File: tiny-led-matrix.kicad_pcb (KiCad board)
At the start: 4 copper layers, 37.5 x 21.2 mm, 166 parts, among them J1 TagConnect_TC2030_SWD, U1 STM32F030F4Px

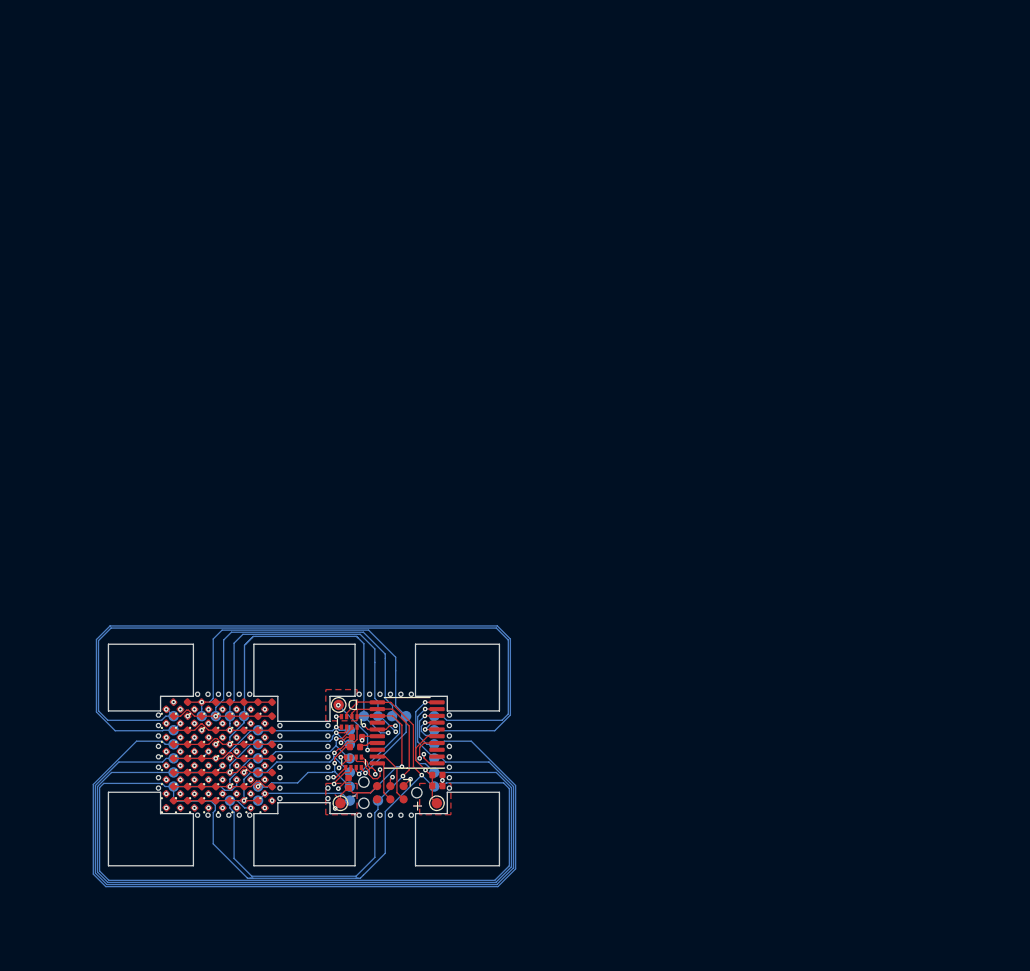
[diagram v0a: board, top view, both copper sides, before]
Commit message: Full panel
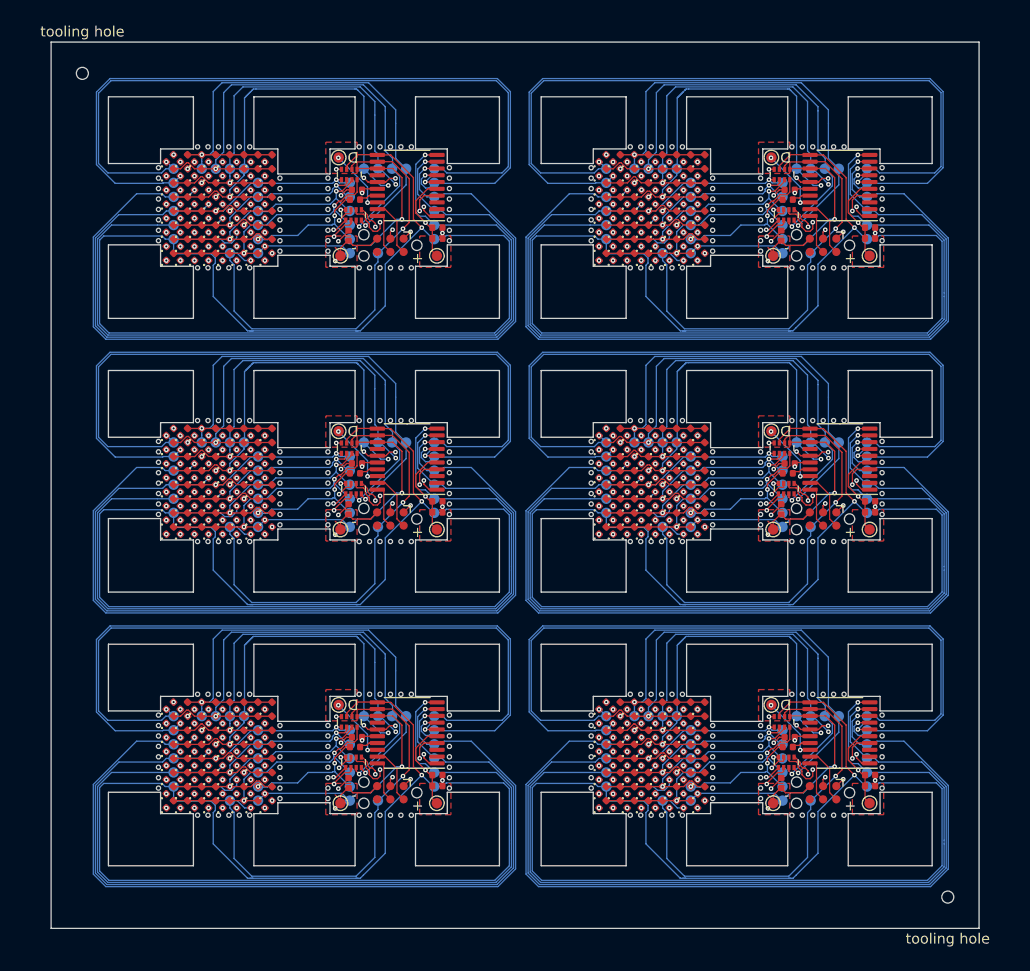
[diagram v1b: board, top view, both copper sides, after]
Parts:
- added C1: 10uF, Capacitor_SMD:C_0402_1005Metric, F.Cu at (167.2, 81.5)
- added C1: 10uF, Capacitor_SMD:C_0402_1005Metric, F.Cu at (167.2, 55.2)
- added C1: 10uF, Capacitor_SMD:C_0402_1005Metric, F.Cu at (167.2, 107.7)
- added C1: 10uF, Capacitor_SMD:C_0402_1005Metric, F.Cu at (125.7, 55.2)
- added C1: 10uF, Capacitor_SMD:C_0402_1005Metric, F.Cu at (125.7, 81.5)
- added C2: 100nF, Capacitor_SMD:C_0402_1005Metric, F.Cu at (159.4, 76.8)
- added C2: 100nF, Capacitor_SMD:C_0402_1005Metric, F.Cu at (159.4, 50.5)
- added C2: 100nF, Capacitor_SMD:C_0402_1005Metric, F.Cu at (159.4, 103.0)
- added C2: 100nF, Capacitor_SMD:C_0402_1005Metric, F.Cu at (117.9, 50.5)
- added C2: 100nF, Capacitor_SMD:C_0402_1005Metric, F.Cu at (117.9, 76.8)
- added C3: 100nF, Capacitor_SMD:C_0402_1005Metric, F.Cu at (167.2, 54.1)
- added C3: 100nF, Capacitor_SMD:C_0402_1005Metric, F.Cu at (167.2, 80.4)
- added C3: 100nF, Capacitor_SMD:C_0402_1005Metric, F.Cu at (167.2, 106.7)
- added C3: 100nF, Capacitor_SMD:C_0402_1005Metric, F.Cu at (125.7, 54.1)
- added C3: 100nF, Capacitor_SMD:C_0402_1005Metric, F.Cu at (125.7, 80.4)
- added C4: 100nF, Capacitor_SMD:C_0402_1005Metric, F.Cu at (158.6, 81.2)
- added C4: 100nF, Capacitor_SMD:C_0402_1005Metric, F.Cu at (158.6, 54.9)
- added C4: 100nF, Capacitor_SMD:C_0402_1005Metric, F.Cu at (158.6, 107.4)
- added C4: 100nF, Capacitor_SMD:C_0402_1005Metric, F.Cu at (117.1, 54.9)
- added C4: 100nF, Capacitor_SMD:C_0402_1005Metric, F.Cu at (117.1, 81.2)
- added D1: LED, LED_SMD:LED_0402_1005Metric, F.Cu at (141.5, 73.8)
- added D1: LED, LED_SMD:LED_0402_1005Metric, F.Cu at (141.5, 47.5)
- added D1: LED, LED_SMD:LED_0402_1005Metric, F.Cu at (141.5, 100.0)
- added D1: LED, LED_SMD:LED_0402_1005Metric, F.Cu at (100.0, 47.5)
- added D1: LED, LED_SMD:LED_0402_1005Metric, F.Cu at (100.0, 73.8)
- added D10: LED, LED_SMD:LED_0402_1005Metric, F.Cu at (142.8, 48.9)
- added D10: LED, LED_SMD:LED_0402_1005Metric, F.Cu at (142.8, 75.1)
- added D10: LED, LED_SMD:LED_0402_1005Metric, F.Cu at (142.8, 101.3)
- added D10: LED, LED_SMD:LED_0402_1005Metric, F.Cu at (101.3, 48.9)
- added D10: LED, LED_SMD:LED_0402_1005Metric, F.Cu at (101.3, 75.1)
- added D11: LED, LED_SMD:LED_0402_1005Metric, F.Cu at (142.8, 50.2)
- added D11: LED, LED_SMD:LED_0402_1005Metric, F.Cu at (142.8, 76.5)
- added D11: LED, LED_SMD:LED_0402_1005Metric, F.Cu at (142.8, 102.7)
- added D11: LED, LED_SMD:LED_0402_1005Metric, F.Cu at (101.3, 50.2)
- added D11: LED, LED_SMD:LED_0402_1005Metric, F.Cu at (101.3, 76.5)
- added D12: LED, LED_SMD:LED_0402_1005Metric, F.Cu at (142.8, 77.8)
- added D12: LED, LED_SMD:LED_0402_1005Metric, F.Cu at (142.8, 51.5)
- added D12: LED, LED_SMD:LED_0402_1005Metric, F.Cu at (142.8, 104.0)
- added D12: LED, LED_SMD:LED_0402_1005Metric, F.Cu at (101.3, 51.5)
- added D12: LED, LED_SMD:LED_0402_1005Metric, F.Cu at (101.3, 77.8)
- added D13: LED, LED_SMD:LED_0402_1005Metric, F.Cu at (142.8, 52.9)
- added D13: LED, LED_SMD:LED_0402_1005Metric, F.Cu at (142.8, 79.2)
- added D13: LED, LED_SMD:LED_0402_1005Metric, F.Cu at (142.8, 105.4)
- added D13: LED, LED_SMD:LED_0402_1005Metric, F.Cu at (101.3, 52.9)
- added D13: LED, LED_SMD:LED_0402_1005Metric, F.Cu at (101.3, 79.2)
- added D14: LED, LED_SMD:LED_0402_1005Metric, F.Cu at (142.8, 54.2)
- added D14: LED, LED_SMD:LED_0402_1005Metric, F.Cu at (142.8, 80.5)
- added D14: LED, LED_SMD:LED_0402_1005Metric, F.Cu at (142.8, 106.8)
- added D14: LED, LED_SMD:LED_0402_1005Metric, F.Cu at (101.3, 54.2)
- added D14: LED, LED_SMD:LED_0402_1005Metric, F.Cu at (101.3, 80.5)
- added D15: LED, LED_SMD:LED_0402_1005Metric, F.Cu at (142.8, 55.6)
- added D15: LED, LED_SMD:LED_0402_1005Metric, F.Cu at (142.8, 81.8)
- added D15: LED, LED_SMD:LED_0402_1005Metric, F.Cu at (142.8, 108.1)
- added D15: LED, LED_SMD:LED_0402_1005Metric, F.Cu at (101.3, 55.6)
- added D15: LED, LED_SMD:LED_0402_1005Metric, F.Cu at (101.3, 81.8)
- added D16: LED, LED_SMD:LED_0402_1005Metric, F.Cu at (142.8, 57.0)
- added D16: LED, LED_SMD:LED_0402_1005Metric, F.Cu at (142.8, 83.2)
- added D16: LED, LED_SMD:LED_0402_1005Metric, F.Cu at (142.8, 109.5)
- added D16: LED, LED_SMD:LED_0402_1005Metric, F.Cu at (101.3, 57.0)
- added D16: LED, LED_SMD:LED_0402_1005Metric, F.Cu at (101.3, 83.2)
- added D17: LED, LED_SMD:LED_0402_1005Metric, F.Cu at (144.2, 47.5)
- added D17: LED, LED_SMD:LED_0402_1005Metric, F.Cu at (144.2, 73.8)
- added D17: LED, LED_SMD:LED_0402_1005Metric, F.Cu at (144.2, 100.0)
- added D17: LED, LED_SMD:LED_0402_1005Metric, F.Cu at (102.7, 47.5)
- added D17: LED, LED_SMD:LED_0402_1005Metric, F.Cu at (102.7, 73.8)
- added D18: LED, LED_SMD:LED_0402_1005Metric, F.Cu at (144.2, 48.9)
- added D18: LED, LED_SMD:LED_0402_1005Metric, F.Cu at (144.2, 75.1)
- added D18: LED, LED_SMD:LED_0402_1005Metric, F.Cu at (144.2, 101.3)
- added D18: LED, LED_SMD:LED_0402_1005Metric, F.Cu at (102.7, 48.9)
- added D18: LED, LED_SMD:LED_0402_1005Metric, F.Cu at (102.7, 75.1)
- added D19: LED, LED_SMD:LED_0402_1005Metric, F.Cu at (144.2, 76.5)
- added D19: LED, LED_SMD:LED_0402_1005Metric, F.Cu at (144.2, 50.2)
- added D19: LED, LED_SMD:LED_0402_1005Metric, F.Cu at (144.2, 102.7)
- added D19: LED, LED_SMD:LED_0402_1005Metric, F.Cu at (102.7, 50.2)
- added D19: LED, LED_SMD:LED_0402_1005Metric, F.Cu at (102.7, 76.5)
- added D2: LED, LED_SMD:LED_0402_1005Metric, F.Cu at (141.5, 75.1)
- added D2: LED, LED_SMD:LED_0402_1005Metric, F.Cu at (141.5, 48.9)
- added D2: LED, LED_SMD:LED_0402_1005Metric, F.Cu at (141.5, 101.3)
- added D2: LED, LED_SMD:LED_0402_1005Metric, F.Cu at (100.0, 48.9)
- added D2: LED, LED_SMD:LED_0402_1005Metric, F.Cu at (100.0, 75.1)
- added D20: LED, LED_SMD:LED_0402_1005Metric, F.Cu at (144.2, 77.8)
- added D20: LED, LED_SMD:LED_0402_1005Metric, F.Cu at (144.2, 51.5)
- added D20: LED, LED_SMD:LED_0402_1005Metric, F.Cu at (144.2, 104.0)
- added D20: LED, LED_SMD:LED_0402_1005Metric, F.Cu at (102.7, 51.5)
- added D20: LED, LED_SMD:LED_0402_1005Metric, F.Cu at (102.7, 77.8)
- added D21: LED, LED_SMD:LED_0402_1005Metric, F.Cu at (144.2, 79.2)
- added D21: LED, LED_SMD:LED_0402_1005Metric, F.Cu at (144.2, 52.9)
- added D21: LED, LED_SMD:LED_0402_1005Metric, F.Cu at (144.2, 105.4)
- added D21: LED, LED_SMD:LED_0402_1005Metric, F.Cu at (102.7, 52.9)
- added D21: LED, LED_SMD:LED_0402_1005Metric, F.Cu at (102.7, 79.2)
- added D22: LED, LED_SMD:LED_0402_1005Metric, F.Cu at (144.2, 54.2)
- added D22: LED, LED_SMD:LED_0402_1005Metric, F.Cu at (144.2, 80.5)
- added D22: LED, LED_SMD:LED_0402_1005Metric, F.Cu at (144.2, 106.8)
- added D22: LED, LED_SMD:LED_0402_1005Metric, F.Cu at (102.7, 54.2)
- added D22: LED, LED_SMD:LED_0402_1005Metric, F.Cu at (102.7, 80.5)
- added D23: LED, LED_SMD:LED_0402_1005Metric, F.Cu at (144.2, 81.8)
- added D23: LED, LED_SMD:LED_0402_1005Metric, F.Cu at (144.2, 55.6)
- added D23: LED, LED_SMD:LED_0402_1005Metric, F.Cu at (144.2, 108.1)
- added D23: LED, LED_SMD:LED_0402_1005Metric, F.Cu at (102.7, 55.6)
- added D23: LED, LED_SMD:LED_0402_1005Metric, F.Cu at (102.7, 81.8)
- added D24: LED, LED_SMD:LED_0402_1005Metric, F.Cu at (144.2, 57.0)
- added D24: LED, LED_SMD:LED_0402_1005Metric, F.Cu at (144.2, 83.2)
- added D24: LED, LED_SMD:LED_0402_1005Metric, F.Cu at (144.2, 109.5)
- added D24: LED, LED_SMD:LED_0402_1005Metric, F.Cu at (102.7, 57.0)
- added D24: LED, LED_SMD:LED_0402_1005Metric, F.Cu at (102.7, 83.2)
- added D25: LED, LED_SMD:LED_0402_1005Metric, F.Cu at (145.6, 73.8)
- added D25: LED, LED_SMD:LED_0402_1005Metric, F.Cu at (145.6, 47.5)
- added D25: LED, LED_SMD:LED_0402_1005Metric, F.Cu at (145.6, 100.0)
- added D25: LED, LED_SMD:LED_0402_1005Metric, F.Cu at (104.0, 47.5)
- added D25: LED, LED_SMD:LED_0402_1005Metric, F.Cu at (104.0, 73.8)
- added D26: LED, LED_SMD:LED_0402_1005Metric, F.Cu at (145.6, 48.9)
- added D26: LED, LED_SMD:LED_0402_1005Metric, F.Cu at (145.6, 75.1)
- added D26: LED, LED_SMD:LED_0402_1005Metric, F.Cu at (145.6, 101.3)
- added D26: LED, LED_SMD:LED_0402_1005Metric, F.Cu at (104.0, 48.9)
- added D26: LED, LED_SMD:LED_0402_1005Metric, F.Cu at (104.0, 75.1)
- added D27: LED, LED_SMD:LED_0402_1005Metric, F.Cu at (145.6, 50.2)
- added D27: LED, LED_SMD:LED_0402_1005Metric, F.Cu at (145.6, 76.5)
- added D27: LED, LED_SMD:LED_0402_1005Metric, F.Cu at (145.6, 102.7)
- added D27: LED, LED_SMD:LED_0402_1005Metric, F.Cu at (104.0, 50.2)
- added D27: LED, LED_SMD:LED_0402_1005Metric, F.Cu at (104.0, 76.5)
- added D28: LED, LED_SMD:LED_0402_1005Metric, F.Cu at (145.6, 77.8)
- added D28: LED, LED_SMD:LED_0402_1005Metric, F.Cu at (145.6, 51.5)
- added D28: LED, LED_SMD:LED_0402_1005Metric, F.Cu at (145.6, 104.0)
- added D28: LED, LED_SMD:LED_0402_1005Metric, F.Cu at (104.0, 51.5)
- added D28: LED, LED_SMD:LED_0402_1005Metric, F.Cu at (104.0, 77.8)
- added D29: LED, LED_SMD:LED_0402_1005Metric, F.Cu at (145.6, 79.2)
- added D29: LED, LED_SMD:LED_0402_1005Metric, F.Cu at (145.6, 52.9)
- added D29: LED, LED_SMD:LED_0402_1005Metric, F.Cu at (145.6, 105.4)
- added D29: LED, LED_SMD:LED_0402_1005Metric, F.Cu at (104.0, 52.9)
- added D29: LED, LED_SMD:LED_0402_1005Metric, F.Cu at (104.0, 79.2)
- added D3: LED, LED_SMD:LED_0402_1005Metric, F.Cu at (141.5, 76.5)
- added D3: LED, LED_SMD:LED_0402_1005Metric, F.Cu at (141.5, 50.2)
- added D3: LED, LED_SMD:LED_0402_1005Metric, F.Cu at (141.5, 102.7)
- added D3: LED, LED_SMD:LED_0402_1005Metric, F.Cu at (100.0, 50.2)
- added D3: LED, LED_SMD:LED_0402_1005Metric, F.Cu at (100.0, 76.5)
- added D30: LED, LED_SMD:LED_0402_1005Metric, F.Cu at (145.6, 80.5)
- added D30: LED, LED_SMD:LED_0402_1005Metric, F.Cu at (145.6, 54.2)
- added D30: LED, LED_SMD:LED_0402_1005Metric, F.Cu at (145.6, 106.8)
- added D30: LED, LED_SMD:LED_0402_1005Metric, F.Cu at (104.0, 54.2)
- added D30: LED, LED_SMD:LED_0402_1005Metric, F.Cu at (104.0, 80.5)
- added D31: LED, LED_SMD:LED_0402_1005Metric, F.Cu at (145.6, 81.8)
- added D31: LED, LED_SMD:LED_0402_1005Metric, F.Cu at (145.6, 55.6)
- added D31: LED, LED_SMD:LED_0402_1005Metric, F.Cu at (145.6, 108.1)
- added D31: LED, LED_SMD:LED_0402_1005Metric, F.Cu at (104.0, 55.6)
- added D31: LED, LED_SMD:LED_0402_1005Metric, F.Cu at (104.0, 81.8)
- added D32: LED, LED_SMD:LED_0402_1005Metric, F.Cu at (145.6, 83.2)
- added D32: LED, LED_SMD:LED_0402_1005Metric, F.Cu at (145.6, 57.0)
- added D32: LED, LED_SMD:LED_0402_1005Metric, F.Cu at (145.6, 109.5)
- added D32: LED, LED_SMD:LED_0402_1005Metric, F.Cu at (104.0, 57.0)
- added D32: LED, LED_SMD:LED_0402_1005Metric, F.Cu at (104.0, 83.2)
- added D33: LED, LED_SMD:LED_0402_1005Metric, F.Cu at (146.9, 73.8)
- added D33: LED, LED_SMD:LED_0402_1005Metric, F.Cu at (146.9, 47.5)
- added D33: LED, LED_SMD:LED_0402_1005Metric, F.Cu at (146.9, 100.0)
- added D33: LED, LED_SMD:LED_0402_1005Metric, F.Cu at (105.4, 47.5)
- added D33: LED, LED_SMD:LED_0402_1005Metric, F.Cu at (105.4, 73.8)
- added D34: LED, LED_SMD:LED_0402_1005Metric, F.Cu at (146.9, 48.9)
- added D34: LED, LED_SMD:LED_0402_1005Metric, F.Cu at (146.9, 75.1)
- added D34: LED, LED_SMD:LED_0402_1005Metric, F.Cu at (146.9, 101.3)
- added D34: LED, LED_SMD:LED_0402_1005Metric, F.Cu at (105.4, 48.9)
- added D34: LED, LED_SMD:LED_0402_1005Metric, F.Cu at (105.4, 75.1)
- added D35: LED, LED_SMD:LED_0402_1005Metric, F.Cu at (146.9, 50.2)
- added D35: LED, LED_SMD:LED_0402_1005Metric, F.Cu at (146.9, 76.5)
- added D35: LED, LED_SMD:LED_0402_1005Metric, F.Cu at (146.9, 102.7)
- added D35: LED, LED_SMD:LED_0402_1005Metric, F.Cu at (105.4, 50.2)
- added D35: LED, LED_SMD:LED_0402_1005Metric, F.Cu at (105.4, 76.5)
- added D36: LED, LED_SMD:LED_0402_1005Metric, F.Cu at (146.9, 77.8)
- added D36: LED, LED_SMD:LED_0402_1005Metric, F.Cu at (146.9, 51.5)
- added D36: LED, LED_SMD:LED_0402_1005Metric, F.Cu at (146.9, 104.0)
- added D36: LED, LED_SMD:LED_0402_1005Metric, F.Cu at (105.4, 51.5)
- added D36: LED, LED_SMD:LED_0402_1005Metric, F.Cu at (105.4, 77.8)
- added D37: LED, LED_SMD:LED_0402_1005Metric, F.Cu at (146.9, 79.2)
- added D37: LED, LED_SMD:LED_0402_1005Metric, F.Cu at (146.9, 52.9)
- added D37: LED, LED_SMD:LED_0402_1005Metric, F.Cu at (146.9, 105.4)
- added D37: LED, LED_SMD:LED_0402_1005Metric, F.Cu at (105.4, 52.9)
- added D37: LED, LED_SMD:LED_0402_1005Metric, F.Cu at (105.4, 79.2)
- added D38: LED, LED_SMD:LED_0402_1005Metric, F.Cu at (146.9, 80.5)
- added D38: LED, LED_SMD:LED_0402_1005Metric, F.Cu at (146.9, 54.2)
- added D38: LED, LED_SMD:LED_0402_1005Metric, F.Cu at (146.9, 106.8)
- added D38: LED, LED_SMD:LED_0402_1005Metric, F.Cu at (105.4, 54.2)
- added D38: LED, LED_SMD:LED_0402_1005Metric, F.Cu at (105.4, 80.5)
- added D39: LED, LED_SMD:LED_0402_1005Metric, F.Cu at (146.9, 81.8)
- added D39: LED, LED_SMD:LED_0402_1005Metric, F.Cu at (146.9, 55.6)
- added D39: LED, LED_SMD:LED_0402_1005Metric, F.Cu at (146.9, 108.1)
- added D39: LED, LED_SMD:LED_0402_1005Metric, F.Cu at (105.4, 55.6)
- added D39: LED, LED_SMD:LED_0402_1005Metric, F.Cu at (105.4, 81.8)
- added D4: LED, LED_SMD:LED_0402_1005Metric, F.Cu at (141.5, 51.5)
- added D4: LED, LED_SMD:LED_0402_1005Metric, F.Cu at (141.5, 77.8)
- added D4: LED, LED_SMD:LED_0402_1005Metric, F.Cu at (141.5, 104.0)
- added D4: LED, LED_SMD:LED_0402_1005Metric, F.Cu at (100.0, 51.5)
- added D4: LED, LED_SMD:LED_0402_1005Metric, F.Cu at (100.0, 77.8)
- added D40: LED, LED_SMD:LED_0402_1005Metric, F.Cu at (146.9, 83.2)
- added D40: LED, LED_SMD:LED_0402_1005Metric, F.Cu at (146.9, 57.0)
- added D40: LED, LED_SMD:LED_0402_1005Metric, F.Cu at (146.9, 109.5)
- added D40: LED, LED_SMD:LED_0402_1005Metric, F.Cu at (105.4, 57.0)
- added D40: LED, LED_SMD:LED_0402_1005Metric, F.Cu at (105.4, 83.2)
- added D41: LED, LED_SMD:LED_0402_1005Metric, F.Cu at (148.2, 47.5)
- added D41: LED, LED_SMD:LED_0402_1005Metric, F.Cu at (148.2, 73.8)
- added D41: LED, LED_SMD:LED_0402_1005Metric, F.Cu at (148.2, 100.0)
- added D41: LED, LED_SMD:LED_0402_1005Metric, F.Cu at (106.8, 47.5)
- added D41: LED, LED_SMD:LED_0402_1005Metric, F.Cu at (106.8, 73.8)
- added D42: LED, LED_SMD:LED_0402_1005Metric, F.Cu at (148.2, 48.9)
- added D42: LED, LED_SMD:LED_0402_1005Metric, F.Cu at (148.2, 75.1)
- added D42: LED, LED_SMD:LED_0402_1005Metric, F.Cu at (148.2, 101.3)
- added D42: LED, LED_SMD:LED_0402_1005Metric, F.Cu at (106.8, 48.9)
- added D42: LED, LED_SMD:LED_0402_1005Metric, F.Cu at (106.8, 75.1)
- added D43: LED, LED_SMD:LED_0402_1005Metric, F.Cu at (148.2, 50.2)
- added D43: LED, LED_SMD:LED_0402_1005Metric, F.Cu at (148.2, 76.5)
- added D43: LED, LED_SMD:LED_0402_1005Metric, F.Cu at (148.2, 102.7)
- added D43: LED, LED_SMD:LED_0402_1005Metric, F.Cu at (106.8, 50.2)
- added D43: LED, LED_SMD:LED_0402_1005Metric, F.Cu at (106.8, 76.5)
- added D44: LED, LED_SMD:LED_0402_1005Metric, F.Cu at (148.2, 77.8)
- added D44: LED, LED_SMD:LED_0402_1005Metric, F.Cu at (148.2, 51.5)
- added D44: LED, LED_SMD:LED_0402_1005Metric, F.Cu at (148.2, 104.0)
- added D44: LED, LED_SMD:LED_0402_1005Metric, F.Cu at (106.8, 51.5)
- added D44: LED, LED_SMD:LED_0402_1005Metric, F.Cu at (106.8, 77.8)
- added D45: LED, LED_SMD:LED_0402_1005Metric, F.Cu at (148.2, 52.9)
- added D45: LED, LED_SMD:LED_0402_1005Metric, F.Cu at (148.2, 79.2)
- added D45: LED, LED_SMD:LED_0402_1005Metric, F.Cu at (148.2, 105.4)
- added D45: LED, LED_SMD:LED_0402_1005Metric, F.Cu at (106.8, 52.9)
- added D45: LED, LED_SMD:LED_0402_1005Metric, F.Cu at (106.8, 79.2)
- added D46: LED, LED_SMD:LED_0402_1005Metric, F.Cu at (148.2, 80.5)
- added D46: LED, LED_SMD:LED_0402_1005Metric, F.Cu at (148.2, 54.2)
- added D46: LED, LED_SMD:LED_0402_1005Metric, F.Cu at (148.2, 106.8)
- added D46: LED, LED_SMD:LED_0402_1005Metric, F.Cu at (106.8, 54.2)
- added D46: LED, LED_SMD:LED_0402_1005Metric, F.Cu at (106.8, 80.5)
- added D47: LED, LED_SMD:LED_0402_1005Metric, F.Cu at (148.2, 81.8)
- added D47: LED, LED_SMD:LED_0402_1005Metric, F.Cu at (148.2, 55.6)
- added D47: LED, LED_SMD:LED_0402_1005Metric, F.Cu at (148.2, 108.1)
- added D47: LED, LED_SMD:LED_0402_1005Metric, F.Cu at (106.8, 55.6)
- added D47: LED, LED_SMD:LED_0402_1005Metric, F.Cu at (106.8, 81.8)
- added D48: LED, LED_SMD:LED_0402_1005Metric, F.Cu at (148.2, 83.2)
- added D48: LED, LED_SMD:LED_0402_1005Metric, F.Cu at (148.2, 57.0)
- added D48: LED, LED_SMD:LED_0402_1005Metric, F.Cu at (148.2, 109.5)
- added D48: LED, LED_SMD:LED_0402_1005Metric, F.Cu at (106.8, 57.0)
- added D48: LED, LED_SMD:LED_0402_1005Metric, F.Cu at (106.8, 83.2)
- added D49: LED, LED_SMD:LED_0402_1005Metric, F.Cu at (149.6, 47.5)
- added D49: LED, LED_SMD:LED_0402_1005Metric, F.Cu at (149.6, 73.8)
- added D49: LED, LED_SMD:LED_0402_1005Metric, F.Cu at (149.6, 100.0)
- added D49: LED, LED_SMD:LED_0402_1005Metric, F.Cu at (108.1, 47.5)
- added D49: LED, LED_SMD:LED_0402_1005Metric, F.Cu at (108.1, 73.8)
- added D5: LED, LED_SMD:LED_0402_1005Metric, F.Cu at (141.5, 52.9)
- added D5: LED, LED_SMD:LED_0402_1005Metric, F.Cu at (141.5, 79.2)
- added D5: LED, LED_SMD:LED_0402_1005Metric, F.Cu at (141.5, 105.4)
- added D5: LED, LED_SMD:LED_0402_1005Metric, F.Cu at (100.0, 52.9)
- added D5: LED, LED_SMD:LED_0402_1005Metric, F.Cu at (100.0, 79.2)
- added D50: LED, LED_SMD:LED_0402_1005Metric, F.Cu at (149.6, 48.9)
- added D50: LED, LED_SMD:LED_0402_1005Metric, F.Cu at (149.6, 75.1)
- added D50: LED, LED_SMD:LED_0402_1005Metric, F.Cu at (149.6, 101.3)
- added D50: LED, LED_SMD:LED_0402_1005Metric, F.Cu at (108.1, 48.9)
- added D50: LED, LED_SMD:LED_0402_1005Metric, F.Cu at (108.1, 75.1)
- added D51: LED, LED_SMD:LED_0402_1005Metric, F.Cu at (149.6, 50.2)
- added D51: LED, LED_SMD:LED_0402_1005Metric, F.Cu at (149.6, 76.5)
- added D51: LED, LED_SMD:LED_0402_1005Metric, F.Cu at (149.6, 102.7)
- added D51: LED, LED_SMD:LED_0402_1005Metric, F.Cu at (108.1, 50.2)
- added D51: LED, LED_SMD:LED_0402_1005Metric, F.Cu at (108.1, 76.5)
- added D52: LED, LED_SMD:LED_0402_1005Metric, F.Cu at (149.6, 51.5)
- added D52: LED, LED_SMD:LED_0402_1005Metric, F.Cu at (149.6, 77.8)
- added D52: LED, LED_SMD:LED_0402_1005Metric, F.Cu at (149.6, 104.0)
- added D52: LED, LED_SMD:LED_0402_1005Metric, F.Cu at (108.1, 51.5)
- added D52: LED, LED_SMD:LED_0402_1005Metric, F.Cu at (108.1, 77.8)
- added D53: LED, LED_SMD:LED_0402_1005Metric, F.Cu at (149.6, 52.9)
- added D53: LED, LED_SMD:LED_0402_1005Metric, F.Cu at (149.6, 79.2)
- added D53: LED, LED_SMD:LED_0402_1005Metric, F.Cu at (149.6, 105.4)
- added D53: LED, LED_SMD:LED_0402_1005Metric, F.Cu at (108.1, 52.9)
- added D53: LED, LED_SMD:LED_0402_1005Metric, F.Cu at (108.1, 79.2)
- added D54: LED, LED_SMD:LED_0402_1005Metric, F.Cu at (149.6, 80.5)
- added D54: LED, LED_SMD:LED_0402_1005Metric, F.Cu at (149.6, 54.2)
- added D54: LED, LED_SMD:LED_0402_1005Metric, F.Cu at (149.6, 106.8)
- added D54: LED, LED_SMD:LED_0402_1005Metric, F.Cu at (108.1, 54.2)
- added D54: LED, LED_SMD:LED_0402_1005Metric, F.Cu at (108.1, 80.5)
- added D55: LED, LED_SMD:LED_0402_1005Metric, F.Cu at (149.6, 81.8)
- added D55: LED, LED_SMD:LED_0402_1005Metric, F.Cu at (149.6, 55.6)
- added D55: LED, LED_SMD:LED_0402_1005Metric, F.Cu at (149.6, 108.1)
- added D55: LED, LED_SMD:LED_0402_1005Metric, F.Cu at (108.1, 55.6)
- added D55: LED, LED_SMD:LED_0402_1005Metric, F.Cu at (108.1, 81.8)
- added D56: LED, LED_SMD:LED_0402_1005Metric, F.Cu at (149.6, 83.2)
- added D56: LED, LED_SMD:LED_0402_1005Metric, F.Cu at (149.6, 109.5)
- added D56: LED, LED_SMD:LED_0402_1005Metric, F.Cu at (149.6, 57.0)
- added D56: LED, LED_SMD:LED_0402_1005Metric, F.Cu at (108.1, 57.0)
- added D56: LED, LED_SMD:LED_0402_1005Metric, F.Cu at (108.1, 83.2)
- added D57: LED, LED_SMD:LED_0402_1005Metric, F.Cu at (150.9, 47.5)
- added D57: LED, LED_SMD:LED_0402_1005Metric, F.Cu at (150.9, 73.8)
- added D57: LED, LED_SMD:LED_0402_1005Metric, F.Cu at (150.9, 100.0)
- added D57: LED, LED_SMD:LED_0402_1005Metric, F.Cu at (109.5, 47.5)
- added D57: LED, LED_SMD:LED_0402_1005Metric, F.Cu at (109.5, 73.8)
- added D58: LED, LED_SMD:LED_0402_1005Metric, F.Cu at (150.9, 48.9)
- added D58: LED, LED_SMD:LED_0402_1005Metric, F.Cu at (150.9, 75.1)
- added D58: LED, LED_SMD:LED_0402_1005Metric, F.Cu at (150.9, 101.3)
- added D58: LED, LED_SMD:LED_0402_1005Metric, F.Cu at (109.5, 48.9)
- added D58: LED, LED_SMD:LED_0402_1005Metric, F.Cu at (109.5, 75.1)
- added D59: LED, LED_SMD:LED_0402_1005Metric, F.Cu at (150.9, 50.2)
- added D59: LED, LED_SMD:LED_0402_1005Metric, F.Cu at (150.9, 76.5)
- added D59: LED, LED_SMD:LED_0402_1005Metric, F.Cu at (150.9, 102.7)
- added D59: LED, LED_SMD:LED_0402_1005Metric, F.Cu at (109.5, 50.2)
- added D59: LED, LED_SMD:LED_0402_1005Metric, F.Cu at (109.5, 76.5)
- added D6: LED, LED_SMD:LED_0402_1005Metric, F.Cu at (141.5, 54.2)
- added D6: LED, LED_SMD:LED_0402_1005Metric, F.Cu at (141.5, 80.5)
- added D6: LED, LED_SMD:LED_0402_1005Metric, F.Cu at (141.5, 106.8)
- added D6: LED, LED_SMD:LED_0402_1005Metric, F.Cu at (100.0, 54.2)
- added D6: LED, LED_SMD:LED_0402_1005Metric, F.Cu at (100.0, 80.5)
- added D60: LED, LED_SMD:LED_0402_1005Metric, F.Cu at (150.9, 77.8)
- added D60: LED, LED_SMD:LED_0402_1005Metric, F.Cu at (150.9, 51.5)
- added D60: LED, LED_SMD:LED_0402_1005Metric, F.Cu at (150.9, 104.0)
- added D60: LED, LED_SMD:LED_0402_1005Metric, F.Cu at (109.5, 51.5)
- added D60: LED, LED_SMD:LED_0402_1005Metric, F.Cu at (109.5, 77.8)
- added D61: LED, LED_SMD:LED_0402_1005Metric, F.Cu at (150.9, 52.9)
- added D61: LED, LED_SMD:LED_0402_1005Metric, F.Cu at (150.9, 79.2)
- added D61: LED, LED_SMD:LED_0402_1005Metric, F.Cu at (150.9, 105.4)
- added D61: LED, LED_SMD:LED_0402_1005Metric, F.Cu at (109.5, 52.9)
- added D61: LED, LED_SMD:LED_0402_1005Metric, F.Cu at (109.5, 79.2)
- added D62: LED, LED_SMD:LED_0402_1005Metric, F.Cu at (150.9, 80.5)
- added D62: LED, LED_SMD:LED_0402_1005Metric, F.Cu at (150.9, 54.2)
- added D62: LED, LED_SMD:LED_0402_1005Metric, F.Cu at (150.9, 106.8)
- added D62: LED, LED_SMD:LED_0402_1005Metric, F.Cu at (109.5, 54.2)
- added D62: LED, LED_SMD:LED_0402_1005Metric, F.Cu at (109.5, 80.5)
- added D63: LED, LED_SMD:LED_0402_1005Metric, F.Cu at (150.9, 81.8)
- added D63: LED, LED_SMD:LED_0402_1005Metric, F.Cu at (150.9, 55.6)
- added D63: LED, LED_SMD:LED_0402_1005Metric, F.Cu at (150.9, 108.1)
- added D63: LED, LED_SMD:LED_0402_1005Metric, F.Cu at (109.5, 55.6)
- added D63: LED, LED_SMD:LED_0402_1005Metric, F.Cu at (109.5, 81.8)
- added D64: LED, LED_SMD:LED_0402_1005Metric, F.Cu at (150.9, 83.2)
- added D64: LED, LED_SMD:LED_0402_1005Metric, F.Cu at (150.9, 57.0)
- added D64: LED, LED_SMD:LED_0402_1005Metric, F.Cu at (150.9, 109.5)
- added D64: LED, LED_SMD:LED_0402_1005Metric, F.Cu at (109.5, 57.0)
- added D64: LED, LED_SMD:LED_0402_1005Metric, F.Cu at (109.5, 83.2)
- added D7: LED, LED_SMD:LED_0402_1005Metric, F.Cu at (141.5, 81.8)
- added D7: LED, LED_SMD:LED_0402_1005Metric, F.Cu at (141.5, 55.6)
- added D7: LED, LED_SMD:LED_0402_1005Metric, F.Cu at (141.5, 108.1)
- added D7: LED, LED_SMD:LED_0402_1005Metric, F.Cu at (100.0, 55.6)
- added D7: LED, LED_SMD:LED_0402_1005Metric, F.Cu at (100.0, 81.8)
- added D8: LED, LED_SMD:LED_0402_1005Metric, F.Cu at (141.5, 57.0)
- added D8: LED, LED_SMD:LED_0402_1005Metric, F.Cu at (141.5, 83.2)
- added D8: LED, LED_SMD:LED_0402_1005Metric, F.Cu at (141.5, 109.5)
- added D8: LED, LED_SMD:LED_0402_1005Metric, F.Cu at (100.0, 57.0)
- added D8: LED, LED_SMD:LED_0402_1005Metric, F.Cu at (100.0, 83.2)
- added D9: LED, LED_SMD:LED_0402_1005Metric, F.Cu at (142.8, 73.8)
- added D9: LED, LED_SMD:LED_0402_1005Metric, F.Cu at (142.8, 47.5)
- added D9: LED, LED_SMD:LED_0402_1005Metric, F.Cu at (142.8, 100.0)
- added D9: LED, LED_SMD:LED_0402_1005Metric, F.Cu at (101.3, 47.5)
- added D9: LED, LED_SMD:LED_0402_1005Metric, F.Cu at (101.3, 73.8)
- added J1: TagConnect_TC2030_SWD, Connector:Tag-Connect_TC2030-IDC-NL_2x03_P1.27mm_Vertical, F.Cu at (162.6, 55.8)
- added J1: TagConnect_TC2030_SWD, Connector:Tag-Connect_TC2030-IDC-NL_2x03_P1.27mm_Vertical, F.Cu at (162.6, 82.1)
- added J1: TagConnect_TC2030_SWD, Connector:Tag-Connect_TC2030-IDC-NL_2x03_P1.27mm_Vertical, F.Cu at (162.6, 108.3)
- added J1: TagConnect_TC2030_SWD, Connector:Tag-Connect_TC2030-IDC-NL_2x03_P1.27mm_Vertical, F.Cu at (121.1, 55.8)
- added J1: TagConnect_TC2030_SWD, Connector:Tag-Connect_TC2030-IDC-NL_2x03_P1.27mm_Vertical, F.Cu at (121.1, 82.1)
- added R1: 1kR, Resistor_SMD:R_0402_1005Metric, F.Cu at (159.2, 77.7)
- added R1: 1kR, Resistor_SMD:R_0402_1005Metric, F.Cu at (159.2, 51.5)
- added R1: 1kR, Resistor_SMD:R_0402_1005Metric, F.Cu at (159.2, 104.0)
- added R1: 1kR, Resistor_SMD:R_0402_1005Metric, F.Cu at (117.8, 51.5)
- added R1: 1kR, Resistor_SMD:R_0402_1005Metric, F.Cu at (117.8, 77.7)
- added REF**: ToolingHole_JLCSMT, ToolingHole:ToolingHole_JLCSMT, F.Cu at (174.6, 118.3)
- added REF**: Perforation_0.4mm, Perforation:Perforation_0.4mm, F.Cu at (168.3, 106.9)
- added REF**: Perforation_0.4mm, Perforation:Perforation_0.4mm, F.Cu at (147.2, 98.9)
- added REF**: Perforation_0.4mm, Perforation:Perforation_0.4mm, F.Cu at (144.2, 98.9)
- added REF**: Perforation_0.4mm, Perforation:Perforation_0.4mm, F.Cu at (160.7, 98.9)
- added REF**: Perforation_0.4mm, Perforation:Perforation_0.4mm, F.Cu at (148.2, 110.5)
- added REF**: Perforation_0.4mm, Perforation:Perforation_0.4mm, F.Cu at (161.7, 98.9)
- added REF**: Perforation_0.4mm, Perforation:Perforation_0.4mm, F.Cu at (163.7, 98.9)
- added REF**: Perforation_0.4mm, Perforation:Perforation_0.4mm, F.Cu at (162.7, 110.5)
- added REF**: Perforation_0.4mm, Perforation:Perforation_0.4mm, F.Cu at (140.4, 105.9)
- added REF**: Perforation_0.4mm, Perforation:Perforation_0.4mm, F.Cu at (144.2, 110.5)
- added REF**: Perforation_0.4mm, Perforation:Perforation_0.4mm, F.Cu at (168.3, 105.9)
- added REF**: Perforation_0.4mm, Perforation:Perforation_0.4mm, F.Cu at (161.7, 72.7)
- added REF**: Perforation_0.4mm, Perforation:Perforation_0.4mm, F.Cu at (162.7, 46.4)
- added REF**: Perforation_0.4mm, Perforation:Perforation_0.4mm, F.Cu at (168.3, 52.4)
- added REF**: Perforation_0.4mm, Perforation:Perforation_0.4mm, F.Cu at (147.2, 84.2)
- added REF**: Perforation_0.4mm, Perforation:Perforation_0.4mm, F.Cu at (163.7, 58.0)
- added REF**: Perforation_0.4mm, Perforation:Perforation_0.4mm, F.Cu at (146.2, 46.4)
- added REF**: Perforation_0.4mm, Perforation:Perforation_0.4mm, F.Cu at (162.7, 58.0)
- added REF**: Perforation_0.4mm, Perforation:Perforation_0.4mm, F.Cu at (163.7, 46.4)
- added REF**: Perforation_0.4mm, Perforation:Perforation_0.4mm, F.Cu at (161.7, 46.4)
- added REF**: Perforation_0.4mm, Perforation:Perforation_0.4mm, F.Cu at (148.2, 58.0)
- added REF**: Perforation_0.4mm, Perforation:Perforation_0.4mm, F.Cu at (160.7, 46.4)
- added REF**: Perforation_0.4mm, Perforation:Perforation_0.4mm, F.Cu at (156.7, 103.9)
- added REF**: Perforation_0.4mm, Perforation:Perforation_0.4mm, F.Cu at (144.2, 46.4)
- added REF**: Perforation_0.4mm, Perforation:Perforation_0.4mm, F.Cu at (147.2, 46.4)
- added REF**: Perforation_0.4mm, Perforation:Perforation_0.4mm, F.Cu at (161.7, 58.0)
- added REF**: Perforation_0.4mm, Perforation:Perforation_0.4mm, F.Cu at (160.7, 58.0)
- added REF**: Perforation_0.4mm, Perforation:Perforation_0.4mm, F.Cu at (164.7, 58.0)
- added REF**: Perforation_0.4mm, Perforation:Perforation_0.4mm, F.Cu at (159.7, 58.0)
- added REF**: Perforation_0.4mm, Perforation:Perforation_0.4mm, F.Cu at (156.7, 81.7)
- added REF**: Perforation_0.4mm, Perforation:Perforation_0.4mm, F.Cu at (152.1, 79.7)
- added REF**: Perforation_0.4mm, Perforation:Perforation_0.4mm, F.Cu at (140.4, 51.4)
- added REF**: Perforation_0.4mm, Perforation:Perforation_0.4mm, F.Cu at (146.2, 58.0)
- added REF**: Perforation_0.4mm, Perforation:Perforation_0.4mm, F.Cu at (156.7, 102.9)
- added REF**: Perforation_0.4mm, Perforation:Perforation_0.4mm, F.Cu at (152.1, 49.4)
- added REF**: Perforation_0.4mm, Perforation:Perforation_0.4mm, F.Cu at (152.1, 55.4)
- added REF**: Perforation_0.4mm, Perforation:Perforation_0.4mm, F.Cu at (152.1, 54.4)
- added REF**: Perforation_0.4mm, Perforation:Perforation_0.4mm, F.Cu at (152.1, 53.4)
- added REF**: Perforation_0.4mm, Perforation:Perforation_0.4mm, F.Cu at (152.1, 56.4)
- added REF**: Perforation_0.4mm, Perforation:Perforation_0.4mm, F.Cu at (156.7, 76.7)
- added REF**: Perforation_0.4mm, Perforation:Perforation_0.4mm, F.Cu at (152.1, 50.4)
- added REF**: Perforation_0.4mm, Perforation:Perforation_0.4mm, F.Cu at (152.1, 51.4)
- added REF**: Perforation_0.4mm, Perforation:Perforation_0.4mm, F.Cu at (140.4, 81.7)
- added REF**: Perforation_0.4mm, Perforation:Perforation_0.4mm, F.Cu at (156.7, 78.7)
- added REF**: Perforation_0.4mm, Perforation:Perforation_0.4mm, F.Cu at (156.7, 108.9)
- added REF**: Perforation_0.4mm, Perforation:Perforation_0.4mm, F.Cu at (168.3, 55.4)
- added REF**: Perforation_0.4mm, Perforation:Perforation_0.4mm, F.Cu at (147.2, 58.0)
- added REF**: Perforation_0.4mm, Perforation:Perforation_0.4mm, F.Cu at (152.1, 82.7)
- added REF**: Perforation_0.4mm, Perforation:Perforation_0.4mm, F.Cu at (164.7, 46.4)
- added REF**: Perforation_0.4mm, Perforation:Perforation_0.4mm, F.Cu at (168.3, 50.4)
- added REF**: Perforation_0.4mm, Perforation:Perforation_0.4mm, F.Cu at (168.3, 53.4)
- added REF**: Perforation_0.4mm, Perforation:Perforation_0.4mm, F.Cu at (145.2, 58.0)
- added REF**: Perforation_0.4mm, Perforation:Perforation_0.4mm, F.Cu at (168.3, 48.4)
- added REF**: Perforation_0.4mm, Perforation:Perforation_0.4mm, F.Cu at (168.3, 49.4)
- added REF**: Perforation_0.4mm, Perforation:Perforation_0.4mm, F.Cu at (147.2, 110.5)
- added REF**: Perforation_0.4mm, Perforation:Perforation_0.4mm, F.Cu at (152.1, 77.7)
- added REF**: Perforation_0.4mm, Perforation:Perforation_0.4mm, F.Cu at (159.7, 46.4)
- added REF**: Perforation_0.4mm, Perforation:Perforation_0.4mm, F.Cu at (140.4, 52.4)
- added REF**: Perforation_0.4mm, Perforation:Perforation_0.4mm, F.Cu at (140.4, 49.4)
- added REF**: Perforation_0.4mm, Perforation:Perforation_0.4mm, F.Cu at (140.4, 50.4)
- added REF**: Perforation_0.4mm, Perforation:Perforation_0.4mm, F.Cu at (156.7, 56.4)
- added REF**: Perforation_0.4mm, Perforation:Perforation_0.4mm, F.Cu at (156.7, 50.4)
- added REF**: Perforation_0.4mm, Perforation:Perforation_0.4mm, F.Cu at (156.7, 51.4)
- added REF**: Perforation_0.4mm, Perforation:Perforation_0.4mm, F.Cu at (168.3, 54.4)
- added REF**: Perforation_0.4mm, Perforation:Perforation_0.4mm, F.Cu at (140.4, 54.4)
- added REF**: Perforation_0.4mm, Perforation:Perforation_0.4mm, F.Cu at (140.4, 55.4)
- added REF**: Perforation_0.4mm, Perforation:Perforation_0.4mm, F.Cu at (168.3, 78.7)
- added REF**: Perforation_0.4mm, Perforation:Perforation_0.4mm, F.Cu at (156.7, 52.4)
- added REF**: Perforation_0.4mm, Perforation:Perforation_0.4mm, F.Cu at (168.3, 51.4)
- added REF**: Perforation_0.4mm, Perforation:Perforation_0.4mm, F.Cu at (144.2, 58.0)
- added REF**: Perforation_0.4mm, Perforation:Perforation_0.4mm, F.Cu at (156.7, 55.4)
- added REF**: Perforation_0.4mm, Perforation:Perforation_0.4mm, F.Cu at (168.3, 77.7)
- added REF**: Perforation_0.4mm, Perforation:Perforation_0.4mm, F.Cu at (168.3, 107.9)
- added REF**: Perforation_0.4mm, Perforation:Perforation_0.4mm, F.Cu at (156.7, 79.7)
- added REF**: Perforation_0.4mm, Perforation:Perforation_0.4mm, F.Cu at (140.4, 103.9)
- added REF**: Perforation_0.4mm, Perforation:Perforation_0.4mm, F.Cu at (168.3, 104.9)
- added REF**: Perforation_0.4mm, Perforation:Perforation_0.4mm, F.Cu at (162.7, 98.9)
- added REF**: Perforation_0.4mm, Perforation:Perforation_0.4mm, F.Cu at (159.7, 72.7)
- added REF**: Perforation_0.4mm, Perforation:Perforation_0.4mm, F.Cu at (156.7, 80.7)
- added REF**: Perforation_0.4mm, Perforation:Perforation_0.4mm, F.Cu at (115.2, 49.4)
- added REF**: Perforation_0.4mm, Perforation:Perforation_0.4mm, F.Cu at (126.8, 51.4)
- added REF**: Perforation_0.4mm, Perforation:Perforation_0.4mm, F.Cu at (115.2, 52.4)
- added REF**: Perforation_0.4mm, Perforation:Perforation_0.4mm, F.Cu at (98.9, 55.4)
- added REF**: Perforation_0.4mm, Perforation:Perforation_0.4mm, F.Cu at (98.9, 54.4)
- added REF**: Perforation_0.4mm, Perforation:Perforation_0.4mm, F.Cu at (126.8, 54.4)
- added REF**: Perforation_0.4mm, Perforation:Perforation_0.4mm, F.Cu at (115.2, 51.4)
- added REF**: Perforation_0.4mm, Perforation:Perforation_0.4mm, F.Cu at (115.2, 50.4)
- added REF**: Perforation_0.4mm, Perforation:Perforation_0.4mm, F.Cu at (115.2, 56.4)
- added REF**: Perforation_0.4mm, Perforation:Perforation_0.4mm, F.Cu at (148.2, 84.2)
- added REF**: Perforation_0.4mm, Perforation:Perforation_0.4mm, F.Cu at (98.9, 50.4)
- added REF**: Perforation_0.4mm, Perforation:Perforation_0.4mm, F.Cu at (98.9, 49.4)
- added REF**: Perforation_0.4mm, Perforation:Perforation_0.4mm, F.Cu at (98.9, 52.4)
- added REF**: Perforation_0.4mm, Perforation:Perforation_0.4mm, F.Cu at (118.2, 46.4)
- added REF**: Perforation_0.4mm, Perforation:Perforation_0.4mm, F.Cu at (126.8, 49.4)
- added REF**: Perforation_0.4mm, Perforation:Perforation_0.4mm, F.Cu at (126.8, 48.4)
- added REF**: Perforation_0.4mm, Perforation:Perforation_0.4mm, F.Cu at (103.7, 58.0)
- added REF**: Perforation_0.4mm, Perforation:Perforation_0.4mm, F.Cu at (126.8, 50.4)
- added REF**: Perforation_0.4mm, Perforation:Perforation_0.4mm, F.Cu at (123.2, 46.4)
- added REF**: Perforation_0.4mm, Perforation:Perforation_0.4mm, F.Cu at (107.7, 58.0)
- added REF**: Perforation_0.4mm, Perforation:Perforation_0.4mm, F.Cu at (160.7, 72.7)
- added REF**: Perforation_0.4mm, Perforation:Perforation_0.4mm, F.Cu at (115.2, 53.4)
- added REF**: Perforation_0.4mm, Perforation:Perforation_0.4mm, F.Cu at (115.2, 54.4)
- added REF**: Perforation_0.4mm, Perforation:Perforation_0.4mm, F.Cu at (115.2, 55.4)
- added REF**: Perforation_0.4mm, Perforation:Perforation_0.4mm, F.Cu at (107.7, 46.4)
- added REF**: Perforation_0.4mm, Perforation:Perforation_0.4mm, F.Cu at (98.9, 48.4)
- added REF**: Perforation_0.4mm, Perforation:Perforation_0.4mm, F.Cu at (103.7, 46.4)
- added REF**: Perforation_0.4mm, Perforation:Perforation_0.4mm, F.Cu at (104.7, 46.4)
- added REF**: Perforation_0.4mm, Perforation:Perforation_0.4mm, F.Cu at (122.2, 58.0)
- added REF**: Perforation_0.4mm, Perforation:Perforation_0.4mm, F.Cu at (106.7, 46.4)
- added REF**: Perforation_0.4mm, Perforation:Perforation_0.4mm, F.Cu at (110.5, 52.4)
- added REF**: ToolingHole_JLCSMT, ToolingHole:ToolingHole_JLCSMT, F.Cu at (91.6, 39.4)
- added REF**: Perforation_0.4mm, Perforation:Perforation_0.4mm, F.Cu at (144.2, 72.7)
- added REF**: Perforation_0.4mm, Perforation:Perforation_0.4mm, F.Cu at (110.5, 51.4)
- added REF**: Perforation_0.4mm, Perforation:Perforation_0.4mm, F.Cu at (110.5, 50.4)
- added REF**: Perforation_0.4mm, Perforation:Perforation_0.4mm, F.Cu at (110.5, 56.4)
- added REF**: Perforation_0.4mm, Perforation:Perforation_0.4mm, F.Cu at (110.5, 53.4)
- added REF**: Perforation_0.4mm, Perforation:Perforation_0.4mm, F.Cu at (110.5, 54.4)
- added REF**: Perforation_0.4mm, Perforation:Perforation_0.4mm, F.Cu at (110.5, 55.4)
- added REF**: Perforation_0.4mm, Perforation:Perforation_0.4mm, F.Cu at (110.5, 49.4)
- added REF**: Perforation_0.4mm, Perforation:Perforation_0.4mm, F.Cu at (104.7, 58.0)
- added REF**: Perforation_0.4mm, Perforation:Perforation_0.4mm, F.Cu at (118.2, 58.0)
- added REF**: Perforation_0.4mm, Perforation:Perforation_0.4mm, F.Cu at (123.2, 58.0)
- added REF**: Perforation_0.4mm, Perforation:Perforation_0.4mm, F.Cu at (152.1, 78.7)
- added REF**: Perforation_0.4mm, Perforation:Perforation_0.4mm, F.Cu at (119.2, 58.0)
- added REF**: Perforation_0.4mm, Perforation:Perforation_0.4mm, F.Cu at (120.2, 58.0)
- added REF**: Perforation_0.4mm, Perforation:Perforation_0.4mm, F.Cu at (105.7, 46.4)
- added REF**: Perforation_0.4mm, Perforation:Perforation_0.4mm, F.Cu at (102.7, 46.4)
- added REF**: Perforation_0.4mm, Perforation:Perforation_0.4mm, F.Cu at (119.2, 46.4)
- added REF**: Perforation_0.4mm, Perforation:Perforation_0.4mm, F.Cu at (106.7, 58.0)
- added REF**: Perforation_0.4mm, Perforation:Perforation_0.4mm, F.Cu at (120.2, 46.4)
- added REF**: Perforation_0.4mm, Perforation:Perforation_0.4mm, F.Cu at (122.2, 46.4)
- added REF**: Perforation_0.4mm, Perforation:Perforation_0.4mm, F.Cu at (121.2, 58.0)
- added REF**: Perforation_0.4mm, Perforation:Perforation_0.4mm, F.Cu at (98.9, 53.4)
- added REF**: Perforation_0.4mm, Perforation:Perforation_0.4mm, F.Cu at (148.2, 72.7)
- added REF**: Perforation_0.4mm, Perforation:Perforation_0.4mm, F.Cu at (102.7, 58.0)
- added REF**: Perforation_0.4mm, Perforation:Perforation_0.4mm, F.Cu at (126.8, 53.4)
- added REF**: Perforation_0.4mm, Perforation:Perforation_0.4mm, F.Cu at (105.7, 58.0)
- added REF**: Perforation_0.4mm, Perforation:Perforation_0.4mm, F.Cu at (126.8, 55.4)
- added REF**: Perforation_0.4mm, Perforation:Perforation_0.4mm, F.Cu at (98.9, 51.4)
- added REF**: Perforation_0.4mm, Perforation:Perforation_0.4mm, F.Cu at (126.8, 52.4)
- added REF**: Perforation_0.4mm, Perforation:Perforation_0.4mm, F.Cu at (121.2, 46.4)
- added REF**: Perforation_0.4mm, Perforation:Perforation_0.4mm, F.Cu at (115.2, 75.7)
- added REF**: Perforation_0.4mm, Perforation:Perforation_0.4mm, F.Cu at (126.8, 77.7)
- added REF**: Perforation_0.4mm, Perforation:Perforation_0.4mm, F.Cu at (115.2, 78.7)
- added REF**: Perforation_0.4mm, Perforation:Perforation_0.4mm, F.Cu at (140.4, 78.7)
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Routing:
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- added copper zone on F.Cu, net (none)
- added copper zone on In1.Cu, net (none)
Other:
- board size 37.5 x 21.2 mm -> 89 x 85 mm
